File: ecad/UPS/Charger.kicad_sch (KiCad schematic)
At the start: 63 parts, among them J1 Barrel_Jack, J2 Conn_01x02_Socket, Q1 Q_PMOS, Q2 Q_PMOS_DGS, Q6 Q_NMOS_GDS, Q7 Q_NMOS_GDS, Q8 Q_NMOS_GDS, Q9 Q_NMOS_GDS, U1 BQ25730RSNR

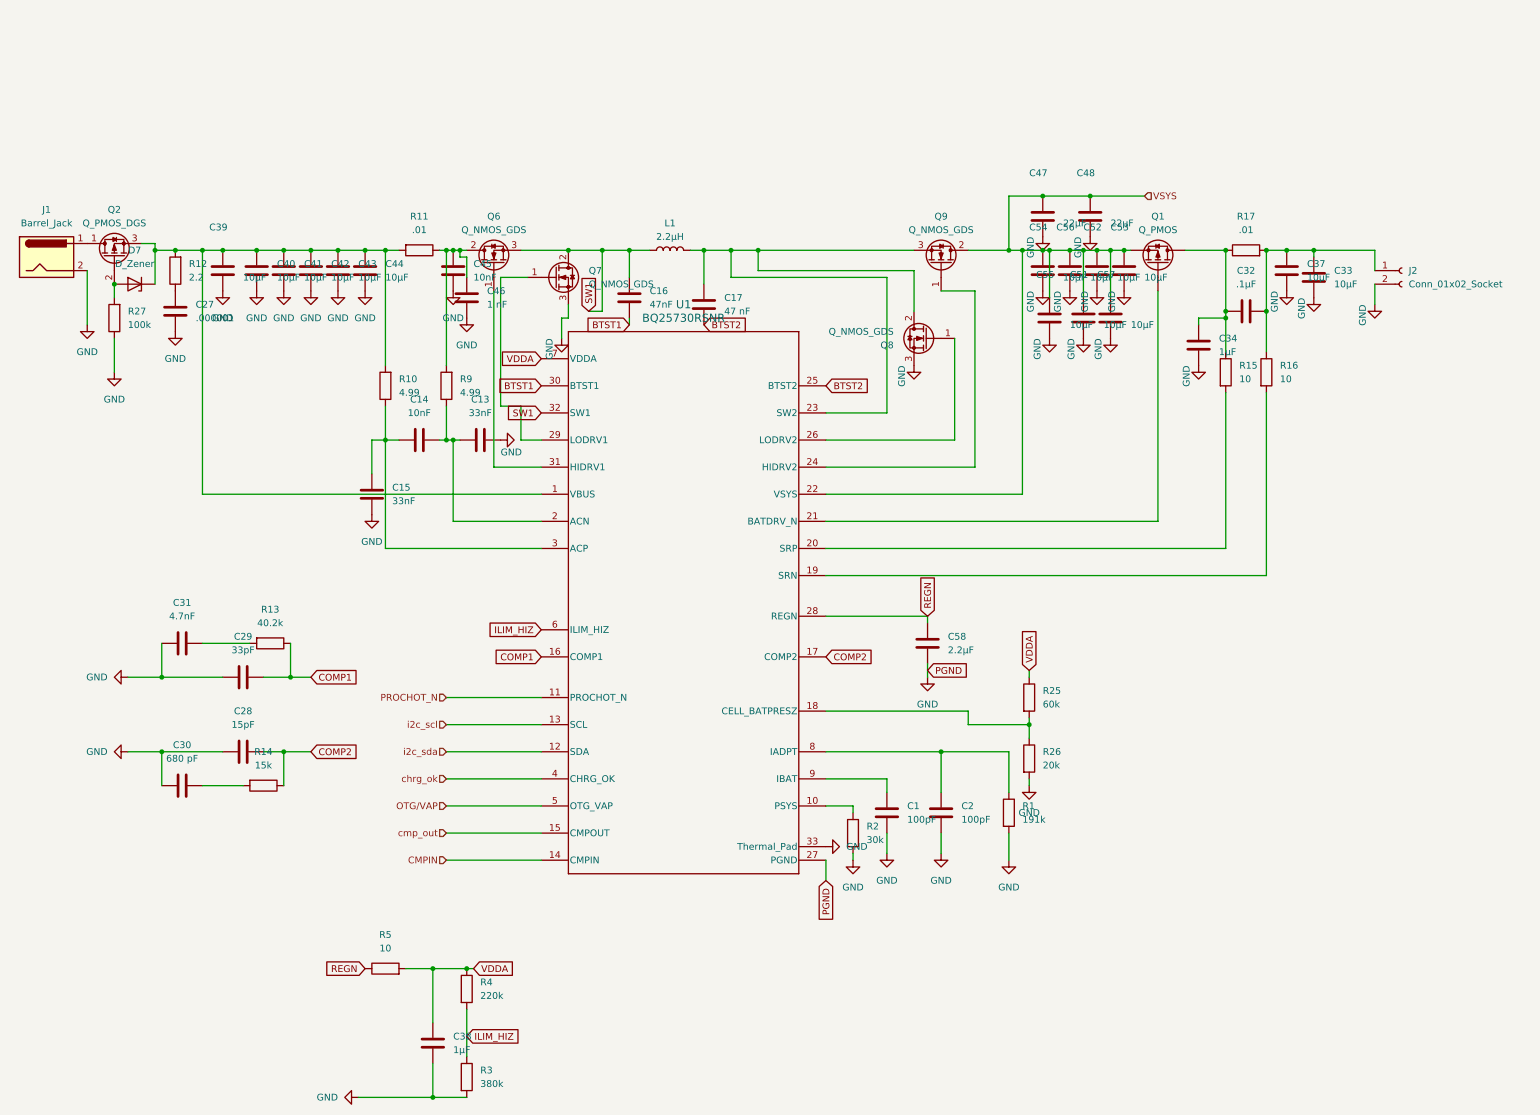
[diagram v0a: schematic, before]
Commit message: More PCB Progress, more to come tomorrow morning
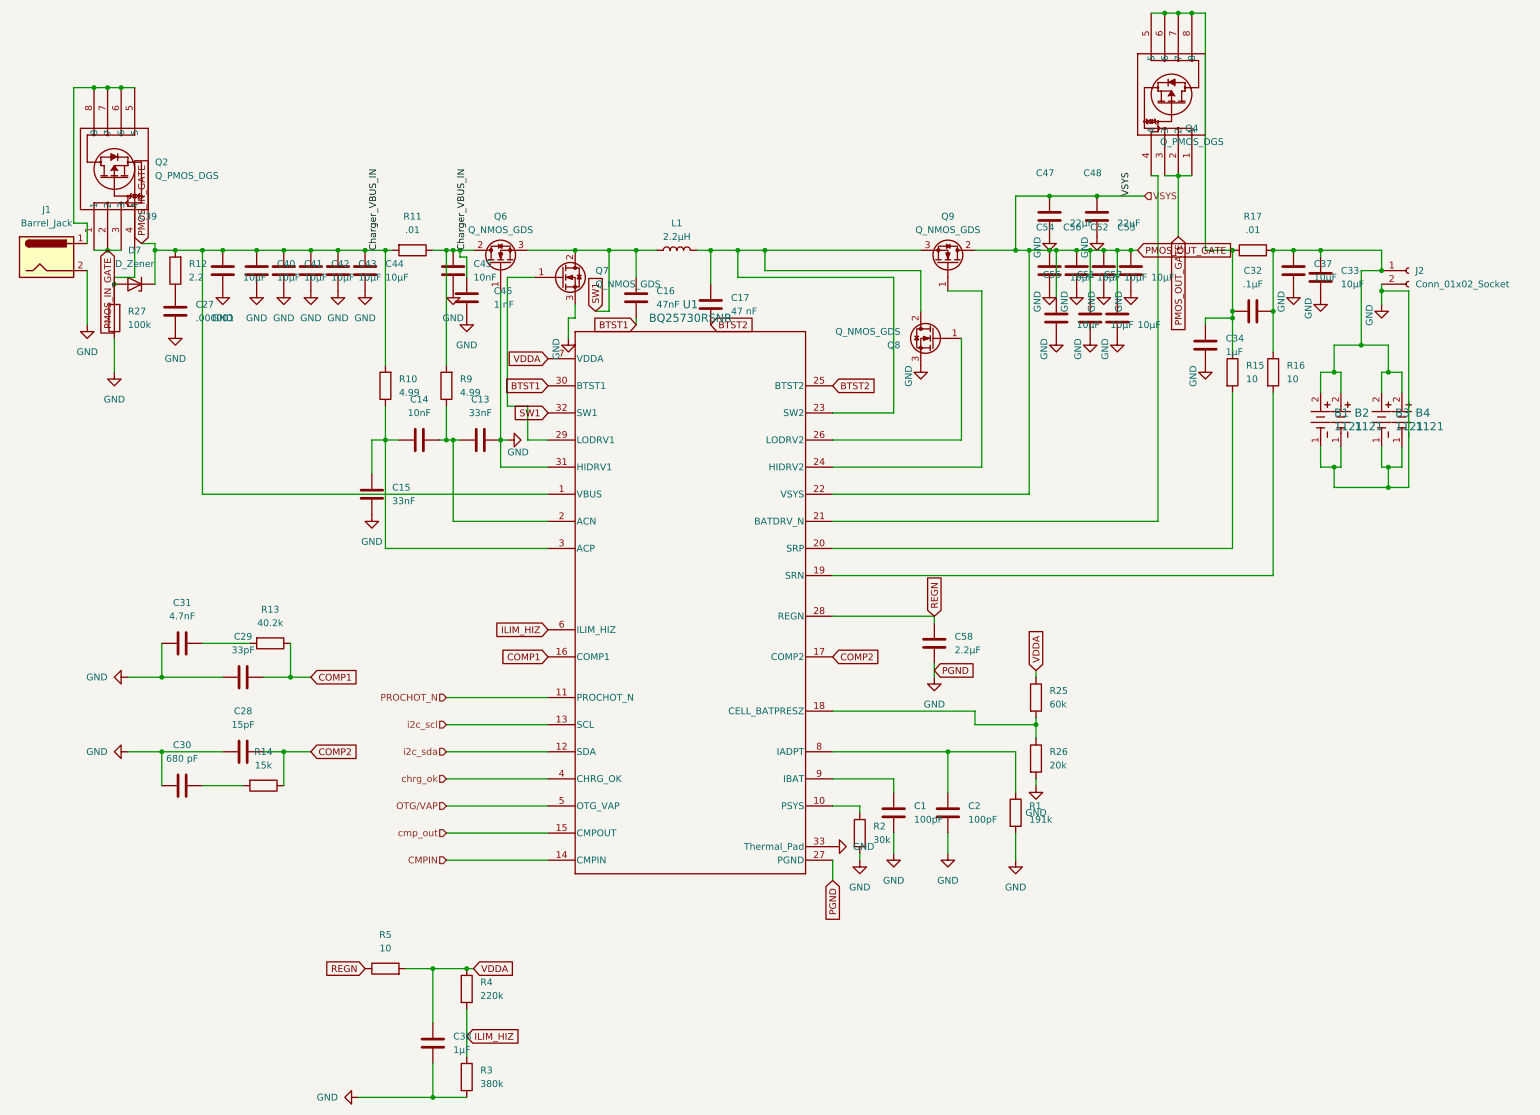
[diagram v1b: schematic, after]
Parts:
- removed Q1: Q_PMOS, UPS:DNK0008A, symbol Device:Q_PMOS
- added B1, B2, B3, B4: 1121, UPS:1121_KEY, symbol UPS:1121
- added Q4: Q_PMOS_DGS, FDS6681Z_OSI, symbol UPS:FDS6681Z
- Q2: footprint UPS:DNK0008A -> FDS6681Z_OSI; symbol Transistor_FET:Q_PMOS_DGS -> UPS:FDS6681Z
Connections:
- net GND: now also Q6.1 (G), U1.31 (HIDRV1), B1.1, B2.1, B3.1, B4.1
- net at C32.1, C33.1, C37.1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: now also B1.2, B2.2, B3.2, B4.2
- net at J1.1: now also Q2.5, Q2.6, Q2.7, Q2.8; no longer Q2.1 (D)
- net at D7.2 (A), R27.2: now also Q2.4; no longer Q2.2 (G)
- net PMOS_IN_GATE: now reaches C39.1, C40.1, C41.1, C42.1, C43.1, C44.1, D7.1 (K), Q2.3, R10.2, R11.2, R12.2, U1.1 (VBUS)
- net PMOS_IN_GATE: now also C45.1, C46.1, Q2.1, Q2.2, Q6.2 (D), R11.1, R9.2
- net at C32.2, C34.1, R15.1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: now also Q4.5, Q4.6, Q4.7, Q4.8
- net at U1.21 (BATDRV_N): now also Q4.4
- net VSYS renamed PMOS_OUT_GATE
- net PMOS_OUT_GATE: now also Q4.1, Q4.2, Q4.3
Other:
- moved on the sheet: C1, C16, C17, C2, C32, C33, C34, C37, C47, C48, C51, C52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
